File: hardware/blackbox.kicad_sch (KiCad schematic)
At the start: 0 parts

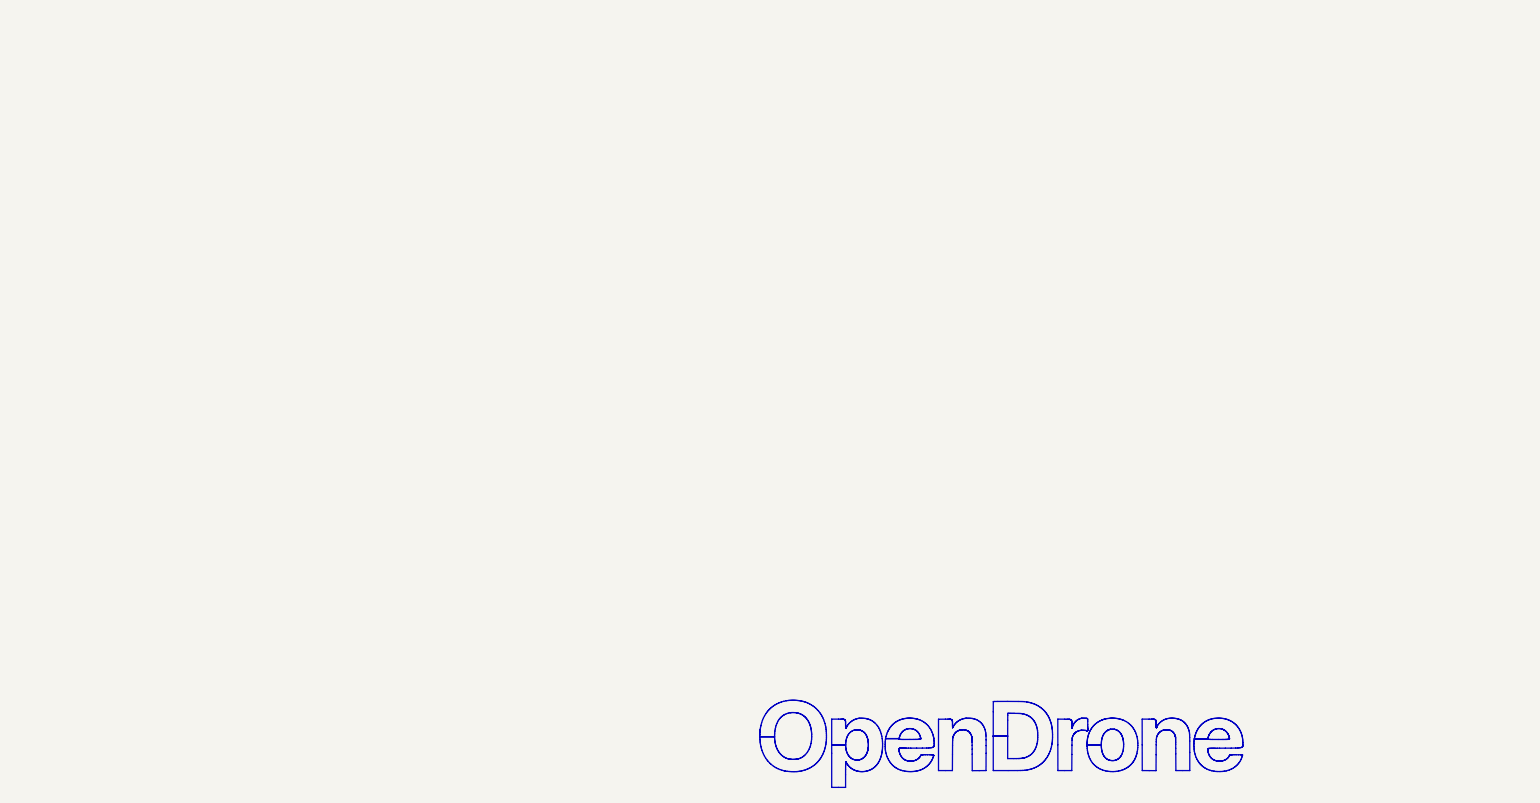
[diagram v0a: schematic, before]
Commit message: wip: schematic sheets in progress
Co-Authored-By: Claude Opus 5.5 <noreply@anthropic.com>
Claude-Session: https://claude.ai/code/session_01RFaS5jnC9tnPam9GBgmGnG
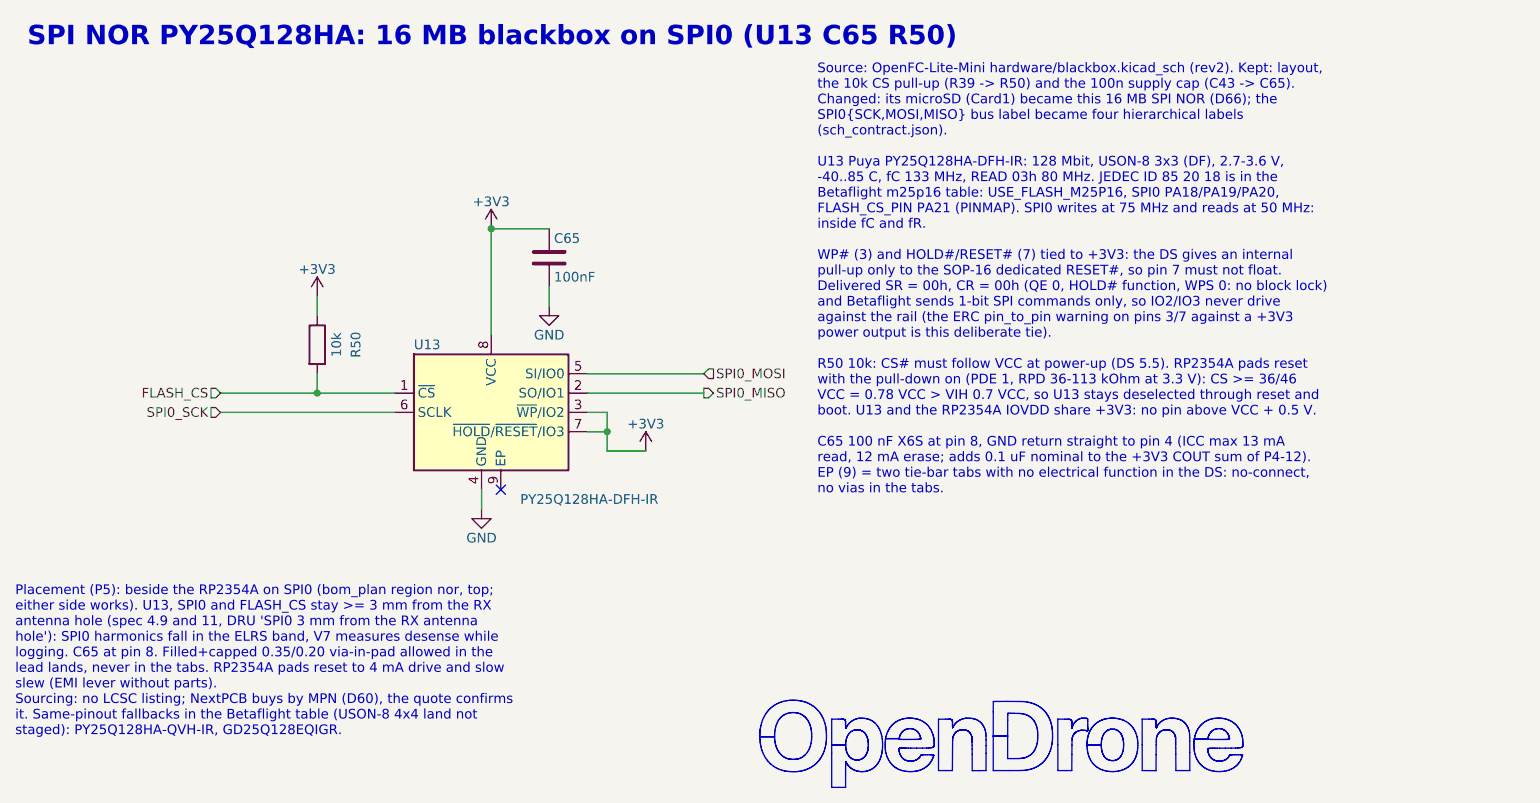
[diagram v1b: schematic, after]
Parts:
- added C65: 100nF, lib:C_0201_0603Metric_W, symbol Device:C
- added R50: 10k, lib:R_0201_0603Metric_W, symbol Device:R
- added U13: PY25Q128HA-DFH-IR, lib:USON-8_3x3mm_P0.8mm_EP_PY25Q128HA, symbol lib:PY25Q128HA-DFH-IR
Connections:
- new net +3V3: C65.1, R50.1, U13.3 (~{WP}/IO2), U13.7 (~{HOLD}/~{RESET}/IO3), U13.8 (VCC)
- new net FLASH_CS: R50.2, U13.1 (~{CS})
- new net GND: C65.2, U13.4 (GND)
- new net SPI0_MISO: U13.2 (SO/IO1)
- new net SPI0_MOSI: U13.5 (SI/IO0)
- new net SPI0_SCK: U13.6 (SCLK)
- no-connect marks 0 -> 1
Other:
- note added: "SPI NOR PY25Q128HA: 16 MB blackbox on SPI0 (U13 C65 R50)"
